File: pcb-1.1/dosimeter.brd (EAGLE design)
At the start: 109 x 61 mm, 54 parts, among them Q1 8Mhz, T1 2N2222, T2 2N2222, T3 2N2907, T4 2n2222, T5 2n2222, T6 2N2907

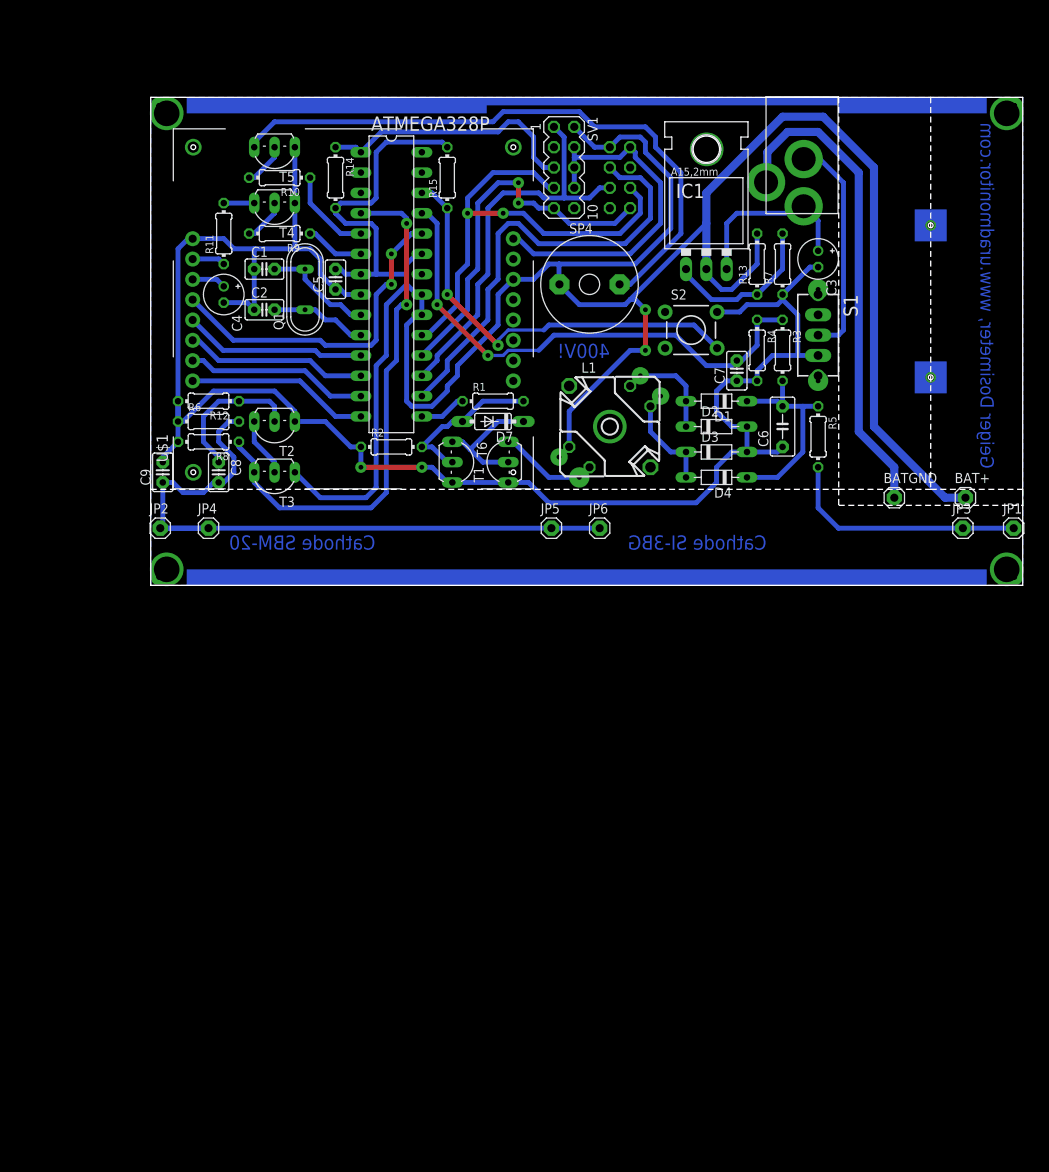
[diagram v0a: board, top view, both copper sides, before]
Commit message: uradmonitor KIT 1.1 update
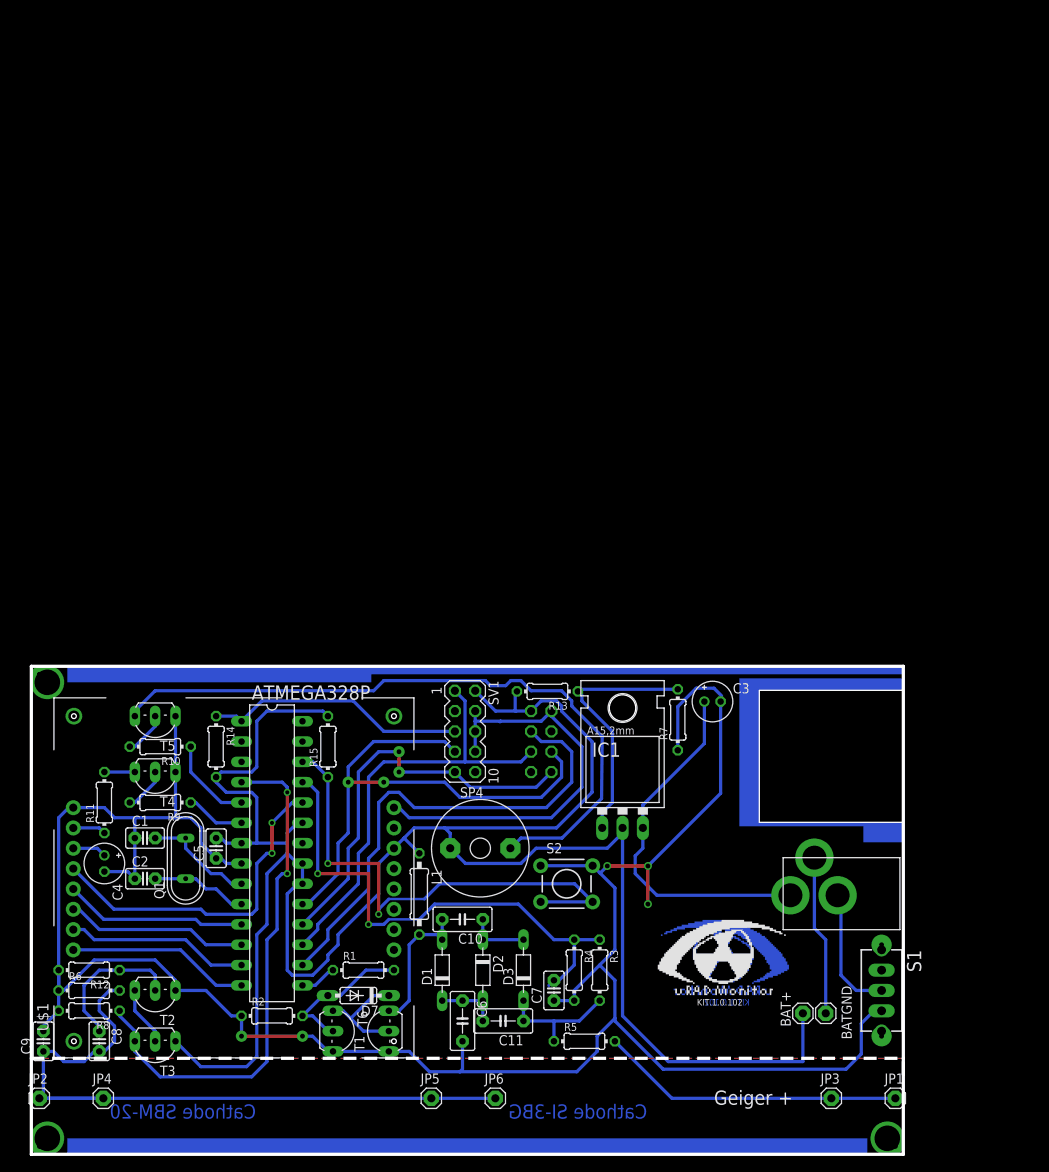
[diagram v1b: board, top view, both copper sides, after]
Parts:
- removed D4: BYV26E, diode:D-7.5
- added C10, C11: 10nF/1KV, capacitor-wima:C5B3
- C6: value 100nF -> 10nF/1KV
- L1: value (none) -> 2.2mH; device trafo-siemens:RM5-4 -> rcl:0207/10
- R13: value 1K -> 2.2K
- R7: value 1.4K -> 3K
- T1: value 2N2222 -> MPSA42
- moved U$2 95.6 mm to (104.3, -28.6), turned to 270 degrees
- moved C6 84.4 mm to (54.0, -44.5), turned to 270 degrees
- moved S1 82.3 mm to (106.4, -40.6)
- moved R5 81.0 mm to (69.2, -47.0), turned to 0 degrees
- moved C7 80.8 mm to (65.4, -40.6)
- moved R3 80.8 mm to (71.1, -38.1)
- moved R4 80.8 mm to (67.9, -38.1)
- moved D1 79.0 mm to (51.4, -38.1), turned to 90 degrees
- moved D2 74.0 mm to (56.5, -38.1), turned to 270 degrees
- moved D7 73.7 mm to (41.0, -41.3)
- moved JP3 73.1 mm to (100.1, -54.1)
- moved R1 72.9 mm to (41.6, -38.1)
- moved JP2 72.9 mm to (1.08, -54.1)
- moved JP5 72.8 mm to (50.1, -54.1)
- moved JP1 72.8 mm to (108.1, -54.1)
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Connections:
- removed net N$12: ATMEGA328P.22, ATMEGA328P.8, C1.1, C2.1, C3.-, C4.-, C5.1, C6.1, C7.1, C9.2, D2.A, D3.A, R12.2, R2.1, R4.2, R6.1, R7.1, R8.2, S1.3, S2.2, SV1.4, SV1.6, SV1.8, SV3.8, T1.E, T2.E, T4.E, T5.E, T6.C, U$1.B8, U$1.T8
- removed net N$32: D3.C, D4.A, L1.3
- removed net N$33: D1.A, D2.C, L1.5
- removed net N$35: C6.2, D1.C, D4.C, R3.2, R5.1
- new net GND: ATMEGA328P.22, ATMEGA328P.8, C1.1, C2.1, C3.-, C4.-, C5.1, C6.2, C7.1, C9.2, R12.2, R2.1, R4.2, R6.1, R7.1, R8.2, S1.3, S2.1, S2.2, SV1.4, SV1.6, SV1.8, SV3.8, T1.E, T2.E, T4.E, T5.E, T6.C, U$1.B8, U$1.T8
- new net N$10: C10.2, D1.A, L1.2, T1.C
- new net N$16: C10.1, D2.C, D3.A
- new net N$30: C11.2, C6.1, D1.C, D2.A
- net N$14: now also S2.3
- net N$25: now also L1.1; no longer L1.6
- net N$31: now also C11.1, D3.C, R3.2, R5.1; no longer L1.2, T1.C
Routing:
- net GND: track 0.00 -> 346.5 mm, vias 0 -> 5
- net N$12: track 264.2 -> 0.00 mm, vias 2 -> 0
- net N$25: track 326.3 -> 270.3 mm, vias 2 -> 0
- net N$20: track 60.9 -> 20.0 mm
- net N$35: track 26.3 -> 0.00 mm
- net N$28: track 22.5 -> 45.6 mm
- net N$10: track 0.00 -> 17.5 mm, vias 1 -> 0
- net N$32: track 13.6 -> 0.00 mm
- net N$33: track 13.1 -> 0.00 mm
- net N$15: track 28.2 -> 16.0 mm
- net N$48: track 20.0 -> 32.2 mm
- net N$14: track 53.7 -> 63.6 mm
- net N$40: track 77.4 -> 86.1 mm
- net N$30: track 0.00 -> 7.62 mm, vias 1 -> 0
- net N$16: track 0.00 -> 7.62 mm, vias 1 -> 0
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- added copper zone on layer 1, net GND
- added copper zone on layer 16, net GND
- removed copper zone on layer 16, net N$77
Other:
- outline, holes or cut-outs redrawn
- board text added: "Geiger +"
- board text added: "KIT.1.0.102"
- board text removed: "400V!"
- board text removed: "Geiger Dosimeter, www.uradmonitor.com"
